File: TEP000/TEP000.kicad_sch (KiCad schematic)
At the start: 25 parts, among them J1 SMA, U1 LT6003HS5#TRMPBF, U2 LT6003HS5#TRMPBF

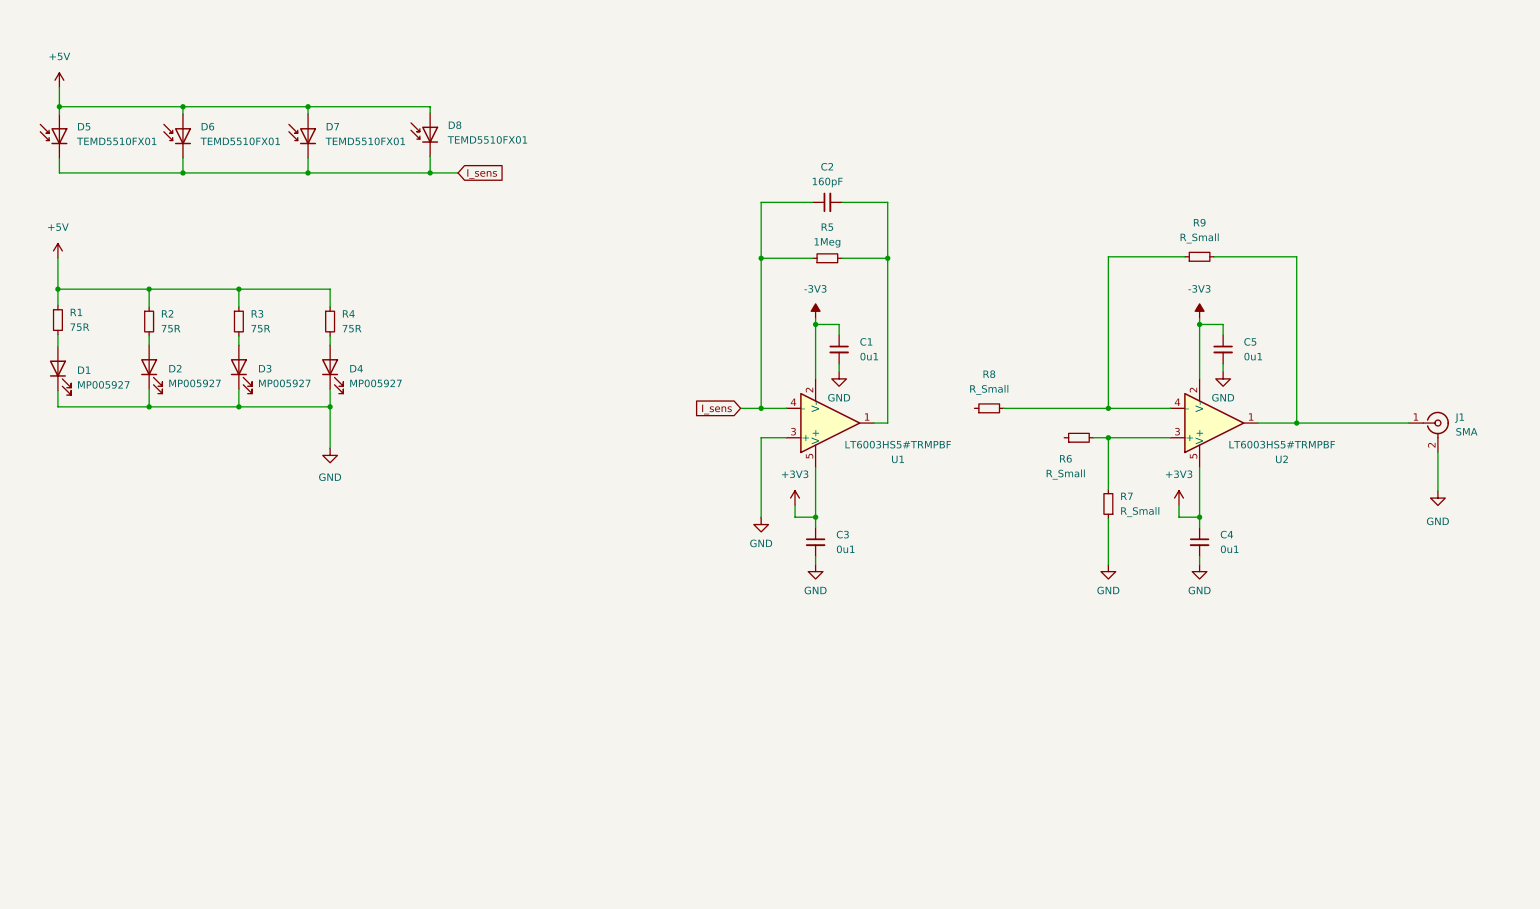
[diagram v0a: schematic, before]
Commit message: First rev of TEP000 Prototype
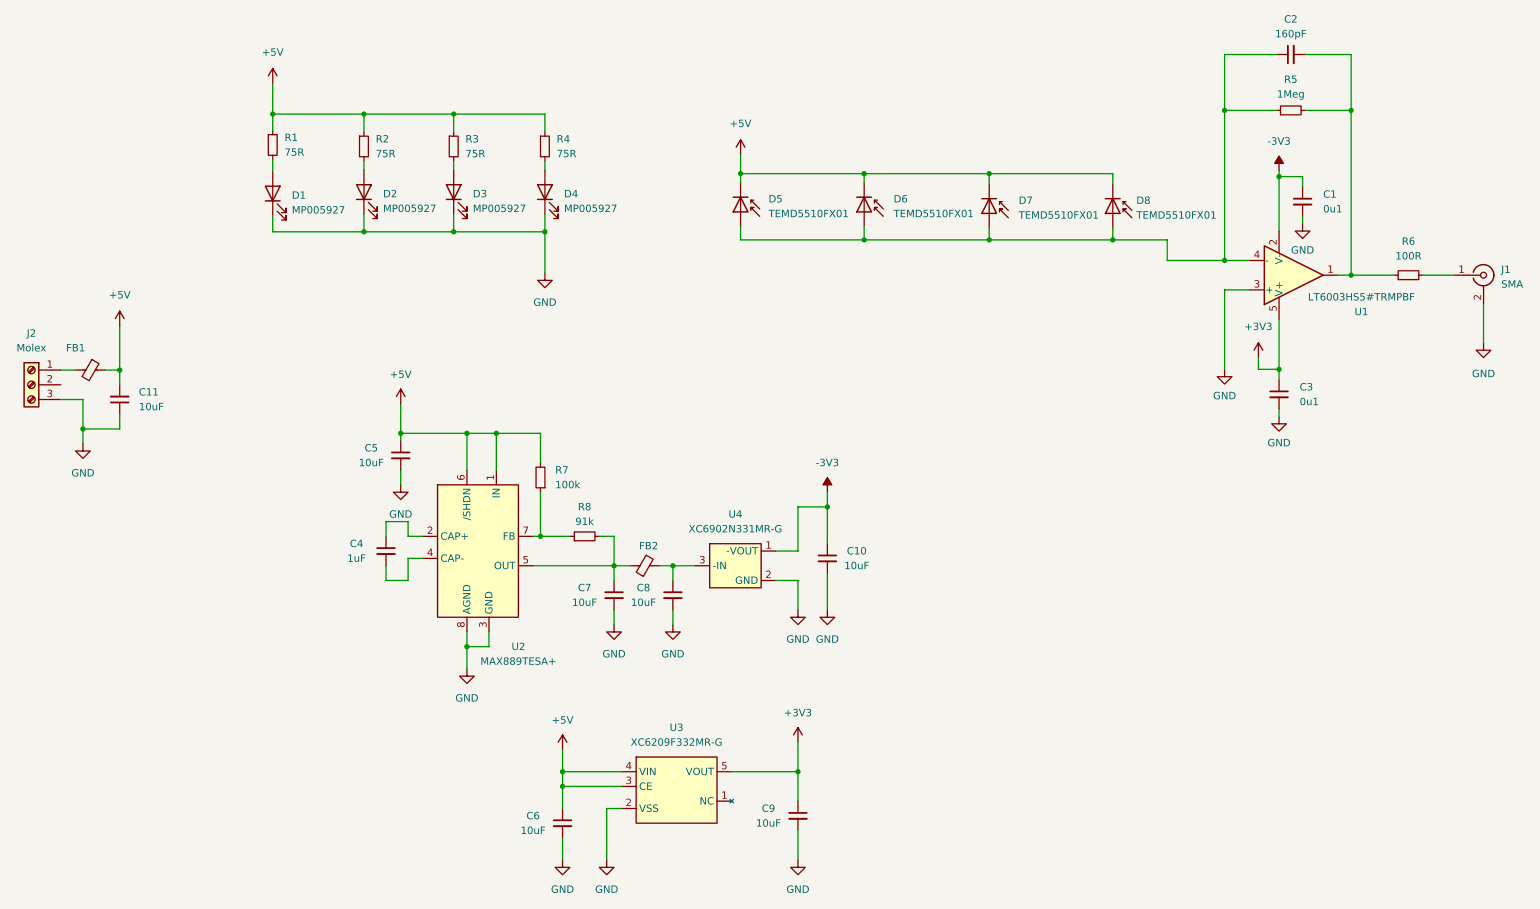
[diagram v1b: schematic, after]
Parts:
- removed R9: R_Small, symbol Device:R_Small
- removed U2: LT6003HS5#TRMPBF, Package_TO_SOT_SMD:SOT-23-5, symbol Amplifier_Operational:LT6015xS5
- added C10, C11, C6, C7, C8, C9: 10uF, Capacitor_SMD:C_0805_2012Metric, symbol Device:C_Small
- added FB1, FB2: MMZ2012Y600BT000, Capacitor_SMD:C_0805_2012Metric_Pad1.18x1.45mm_HandSolder, symbol Device:FerriteBead_Small
- added J2: Molex, MyFootPrints:Screwterminal_3mm81_3pos, symbol Connector:Screw_Terminal_01x03
- added U2: MAX889TESA+, Package_SO:SO-8_3.9x4.9mm_P1.27mm, symbol MySymbols:MAX889TESA+
- added U3: XC6209F332MR-G, Package_TO_SOT_SMD:SOT-89-5, symbol MySymbols:XC6209F332MR-G
- added U4: XC6902N331MR-G, Package_TO_SOT_SMD:SOT-23_Handsoldering, symbol MySymbols:XC6902N331MR-G
- C1, C2, C3: footprint (none) -> Capacitor_SMD:C_0805_2012Metric
- C4: value 0u1 -> 1uF; footprint (none) -> Capacitor_SMD:C_0805_2012Metric
- C5: value 0u1 -> 10uF; footprint (none) -> Capacitor_SMD:C_0805_2012Metric
- D1, D2, D3, D4: footprint (none) -> Diode_SMD:D_0603_1608Metric
- D5, D6, D7, D8: footprint (none) -> MyFootPrints:TEMD5510FX01
- J1: footprint (none) -> Connector_Coaxial:SMA_Amphenol_901-143_Horizontal
- R1, R2, R3, R4, R5: footprint (none) -> Resistor_SMD:R_0805_2012Metric
- R6: value R_Small -> 100R; footprint (none) -> Resistor_SMD:R_0805_2012Metric
- R7: value R_Small -> 100k; footprint (none) -> Resistor_SMD:R_0805_2012Metric
- R8: value R_Small -> 91k; footprint (none) -> Resistor_SMD:R_0805_2012Metric
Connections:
- net +3V3: now also C9.1, U3.5 (VOUT); no longer C4.1
- net +5V: now also C5.1, D5.1 (K), D6.1 (K), D7.1 (K), D8.1 (K), R7.2, C11.2, C6.1, FB1.1, U2.1 (IN), U2.6 (/SHDN), U3.3 (CE), U3.4 (VIN); no longer D5.2 (A), D6.2 (A), D7.2 (A), D8.2 (A)
- net -3V3: now also C10.1, U4.1 (-VOUT); no longer C5.1
- net GND: now also C10.2, C11.1, C6.2, C7.2, C8.2, C9.2, J2.3 (Pin_3), U2.3 (GND), U2.8 (AGND), U3.2 (VSS), U4.2 (GND); no longer C4.2, R7.1
- net at C2.2, R5.2, U1.1: now also R6.1
- net at J1.1 (In): now also R6.2
- net at R8.2: now also C7.1, FB2.1, U2.5 (OUT)
- net at R8.1: now also R7.1, U2.7 (FB)
- removed net I_sens: C2.1, D5.1 (K), D6.1 (K), D7.1 (K), D8.1 (K), R5.1, U1.4 (-)
- new net: C8.1, FB2.2, U4.3 (-IN)
- new net: C4.1, U2.2 (CAP+)
- new net: C4.2, U2.4 (CAP-)
- new net: C2.1, D5.2 (A), D6.2 (A), D7.2 (A), D8.2 (A), R5.1, U1.4 (-)
- new net: FB1.2, J2.1 (Pin_1)
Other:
- moved on the sheet: C1, C2, C3, D1, D2, D3, D4, D5, D6, D7, D8, J1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
